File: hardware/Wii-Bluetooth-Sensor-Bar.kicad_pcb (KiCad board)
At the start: 2 copper layers, 32 x 35 mm, 14 parts, among them J1 LED_Left, J2 LED_Right, SW1 SW_Push, U1 J27H002, U2 LM1117-3.3

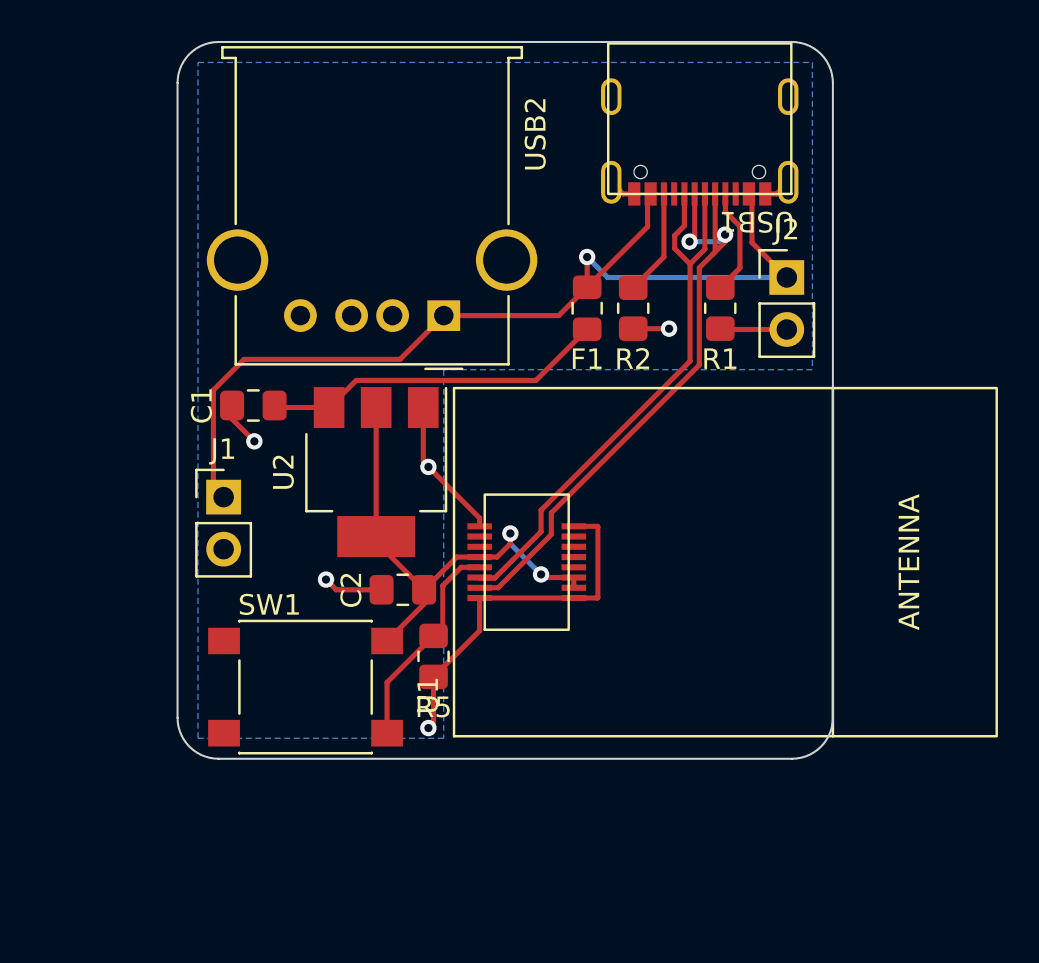
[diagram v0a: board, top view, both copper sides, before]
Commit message: Update schematic/PCB
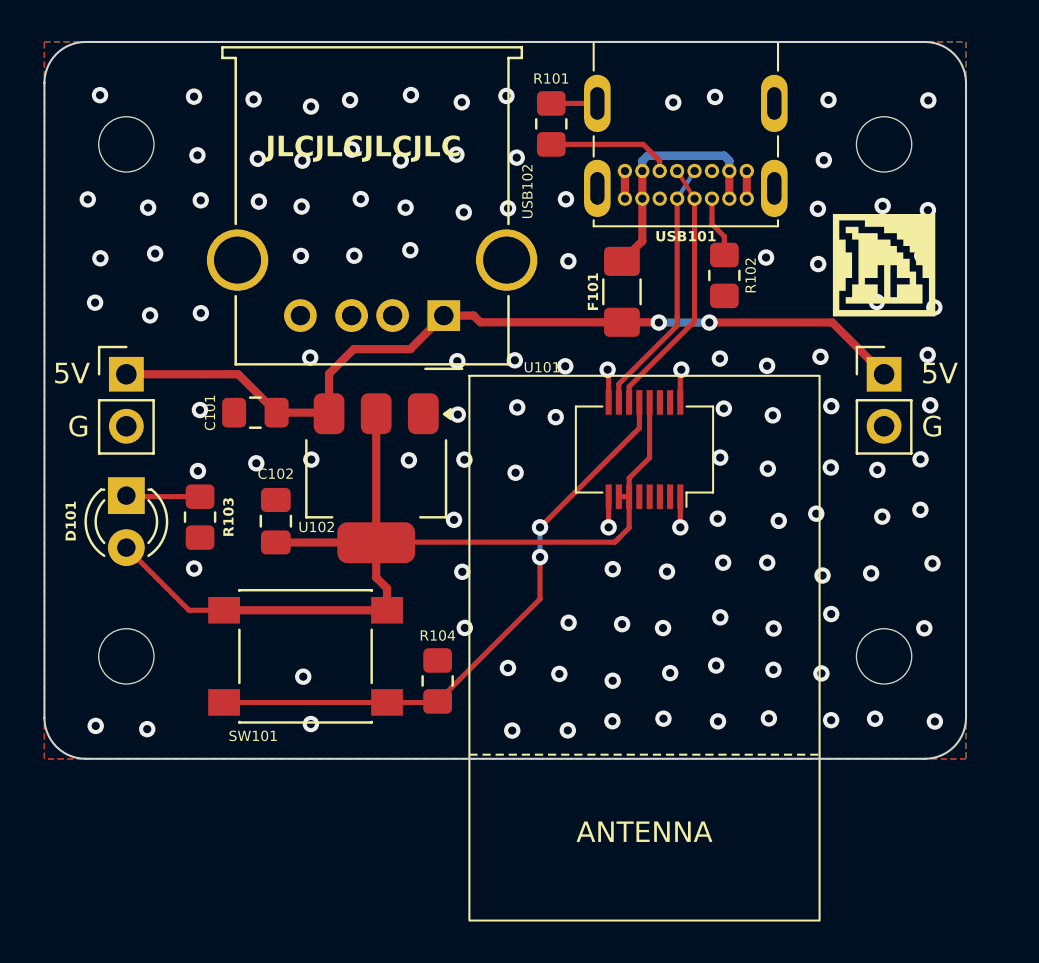
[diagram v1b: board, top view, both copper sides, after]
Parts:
- removed the G*** at (149.2, 105.0)
- removed USB1: USB_C_Receptacle_USB2.0, Amphenol:USB_C_Receptacle_Amphenol_C12402012
- added D101: PWR_GOOD, LED_THT:LED_D3.0mm, F.Cu at (120.5, 98.2)
- added G***: LOGO, Logos:Embedded-Shark-Logo-5mm, F.Cu at (157.5, 86.9)
- added H101: M2.5, MountingHole:MountingHole_2.7mm_M2.5, F.Cu at (120.5, 81.0)
- added H102: M2.5, MountingHole:MountingHole_2.7mm_M2.5, F.Cu at (157.5, 81.0)
- added H103: M2.5, MountingHole:MountingHole_2.7mm_M2.5, F.Cu at (120.5, 106.0)
- added H104: M2.5, MountingHole:MountingHole_2.7mm_M2.5, F.Cu at (157.5, 106.0)
- added R103: 220, Resistor_SMD:R_0805_2012Metric_Pad1.20x1.40mm_HandSolder, F.Cu at (124.1, 99.2)
- added USB101: USB_C_Receptacle_USB2.0, Amphenol:GSB1C211110DS1HR, F.Cu at (147.8, 79.0)
- F101: renamed from F1; footprint Fuse:Fuse_0805_2012Metric_Pad1.15x1.40mm_HandSolder -> Fuse:Fuse_1206_3216Metric_Pad1.42x1.75mm_HandSolder
- R101: renamed from R2; value 5.1K -> 5.1k
- R102: renamed from R1; value 5.1K -> 5.1k
- R104: renamed from R5; value 10K -> 10k
- SW101: renamed from SW1; value SW_Push -> SYNC
- moved U101 11.4 mm to (144.1, 93.6), turned to 0 degrees
- moved R101 9.85 mm to (141.2, 80.0)
- moved J101 7.65 mm to (120.5, 92.2)
- moved C102 7.05 mm to (127.8, 99.4), turned to 90 degrees
- moved J102 6.70 mm to (157.5, 92.2)
- moved F101 1.88 mm to (144.7, 88.2)
- moved R102 1.61 mm to (149.7, 87.4)
- moved SW101 1.50 mm to (129.2, 106.0)
- moved R104 1.22 mm to (135.7, 107.2), turned to 90 degrees
- moved C101 0.36 mm to (126.8, 94.1)
- moved U102 0.30 mm to (132.7, 97.3)
- renumbered C1 to C101, C2 to C102, J1 to J101, J2 to J102, U1 to U101, U2 to U102, USB2 to USB102
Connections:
- C101 pad 1: Net-(U2-VI) -> +5V
- F101 pad 1: +5V -> VBUS
- F101 pad 2: Net-(U2-VI) -> +5V
- R101 pad 1: Net-(USB1-CC2) -> GND
- R101 pad 2: GND -> Net-(USB101-CC2)
- U101 pad 14: (no net) -> unconnected-(U101-Pad14)
- U101 pad 15: (no net) -> unconnected-(U101-Pad15)
- U101 pad 2: (no net) -> unconnected-(U101-Pad2)
- U101 pad 3: (no net) -> unconnected-(U101-Pad3)
- U101 pad 4: (no net) -> unconnected-(U101-Pad4)
- U101 pad 5: (no net) -> unconnected-(U101-Pad5)
- U102 pad 3: Net-(U2-VI) -> +5V
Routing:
- net GND: track 37.4 -> 11.2 mm, vias 5 -> 122
- net +3V3: track 23.5 -> 48.7 mm, vias 2 -> 0
- net Net-(U101-DATA1): track 30.1 -> 11.1 mm, vias 2 -> 0
- net Net-(U101-SYNC): track 10.5 -> 29.1 mm, vias 0 -> 2
- net Net-(U2-VI): track 16.9 -> 0.00 mm
- net Net-(U101-DATA2): track 27.7 -> 11.3 mm
- net VBUS: track 0.00 -> 11.6 mm
- net Net-(USB101-CC2): track 0.00 -> 6.12 mm
- net +5V: track 48.0 -> 42.2 mm, vias 1 -> 2
- net Net-(USB1-CC2): track 5.20 -> 0.00 mm
- net Net-(D101-K): track 0.00 -> 3.62 mm
- net Net-(USB101-CC1): track 5.27 -> 3.00 mm
- added copper zone on F.Cu, net GND
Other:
- board size 32 x 35 mm -> 45 x 35 mm
- board text added: "${PROJECTNAME} REV.${REVISION} ${COMPANY} ${ISSUE_DATE}"
- board text added: "5V"
- board text added: "G"
- board text added: "JLCJLCJLCJLC"
- board text removed: "Wii BT Sensor Bar Revision 1.1 Benjamin Owen"
